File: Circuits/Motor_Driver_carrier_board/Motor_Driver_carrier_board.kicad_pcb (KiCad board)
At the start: 2 copper layers, 35 x 55.6 mm, 21 parts, among them P2 61301021021

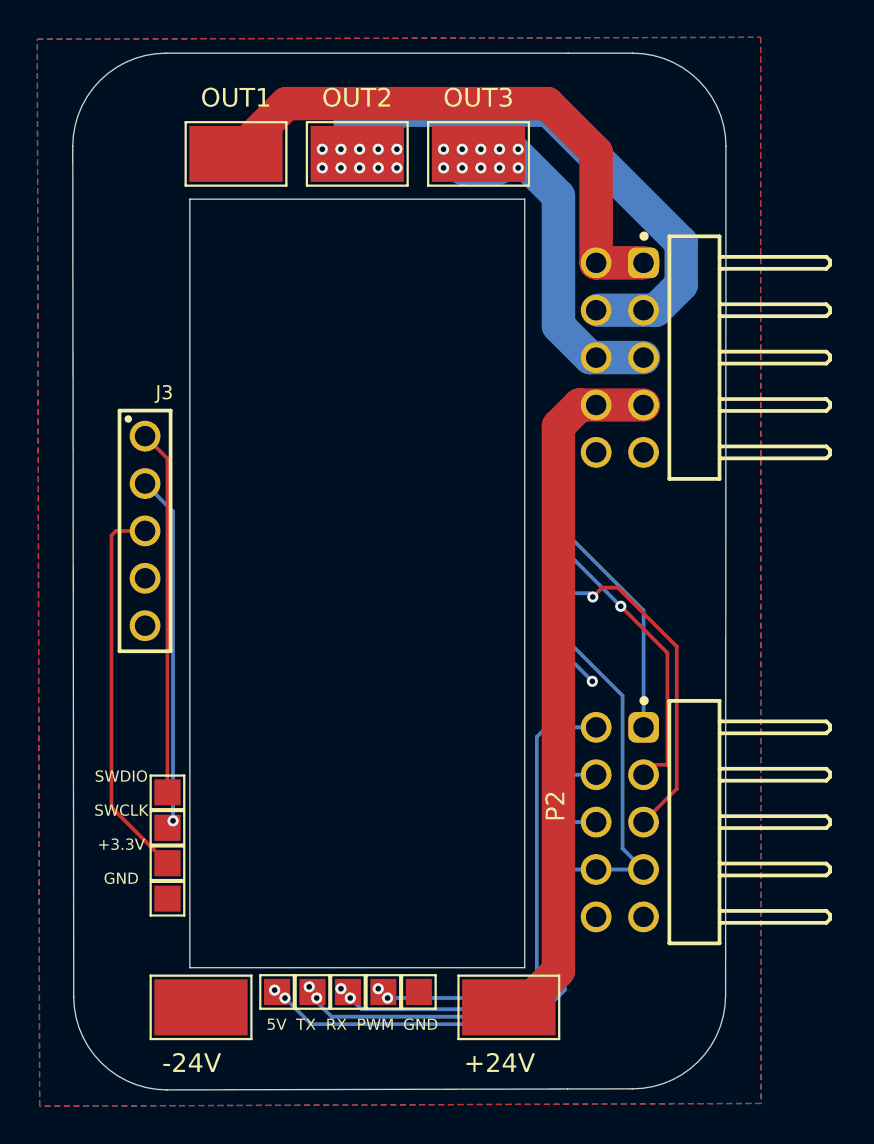
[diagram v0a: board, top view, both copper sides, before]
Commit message: Step file for mainboard pcb updated layout
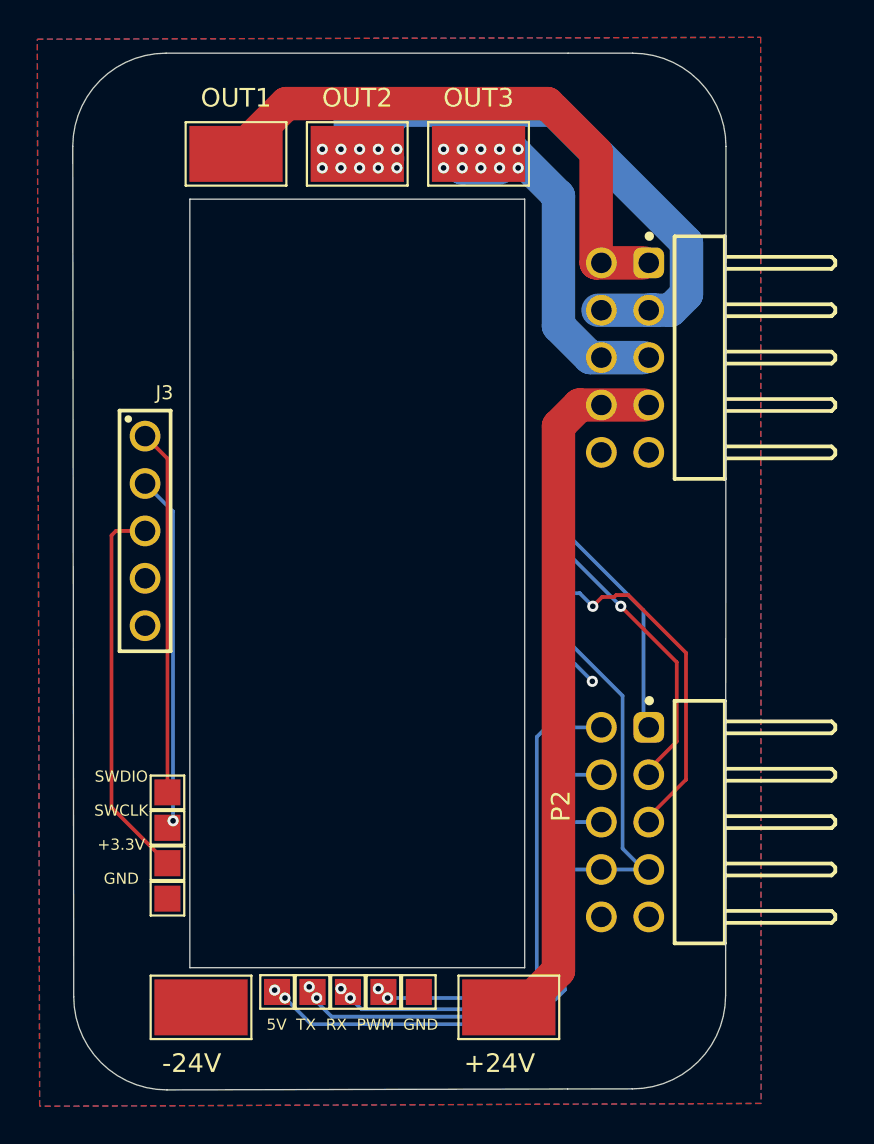
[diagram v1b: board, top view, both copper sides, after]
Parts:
- moved P2 0.28 mm to (151.2, 69.7)
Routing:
- net /OUT2: track 38.9 -> 40.2 mm
- net /H3: track 18.3 -> 18.8 mm
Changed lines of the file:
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@@
 	(footprint "61301021021:ESC_Adapter_pins_right_angle"
 		(layer "F.Cu")
-		(at 150.92 69.65 90)
+		(at 151.2 69.65 90)
 		(descr "Pin Header, pitch 2.54 mm, THT, Angled, dual row, 10p")
 		(property "Reference" "P2"
@@
 		)
 	)
-	(gr_rect
-		(start 118.85 41.34)
-		(end 153.89 97.2)
-		(stroke
-			(width 0.5)
-			(type default)
-		)
-		(fill none)
-		(layer "Eco1.User")
-	)
 	(gr_line
 		(start 148.92 97.07)
@@
 	)
 	(segment
-		(start 134.3 46.7)
-		(end 133.3 46.7)
+		(start 151.82083 54.475896)
+		(end 151.82083 51.711308)
+		(width 1.79166)
+		(layer "B.Cu")
+		(net 3)
+	)
+	(segment
+		(start 151.82083 51.711308)
+		(end 144.717862 44.60834)
 		(width 1.79166)
 		(layer "B.Cu")
@@
 	(segment
 		(start 134.3 46.7)
-		(end 136.39166 44.60834)
+		(end 133.3 46.7)
 		(width 1.79166)
 		(layer "B.Cu")
@@
 	)
 	(segment
-		(start 133.8 44.6)
-		(end 133.8 46.2)
+		(start 144.717862 44.60834)
+		(end 136.39166 44.60834)
 		(width 1.79166)
 		(layer "B.Cu")
@@
 	)
 	(segment
-		(start 151.54083 51.711308)
-		(end 151.54083 53.95917)
+		(start 134.3 46.7)
+		(end 136.39166 44.60834)
 		(width 1.79166)
 		(layer "B.Cu")
@@
 	)
 	(segment
-		(start 151.54083 53.95917)
-		(end 150.17 55.33)
+		(start 133.8 44.6)
+		(end 133.8 46.2)
 		(width 1.79166)
 		(layer "B.Cu")
@@
 	)
 	(segment
-		(start 144.437862 44.60834)
-		(end 151.54083 51.711308)
+		(start 150.966726 55.33)
+		(end 151.82083 54.475896)
 		(width 1.79166)
 		(layer "B.Cu")
@@
 	)
 	(segment
-		(start 136.39166 44.60834)
-		(end 144.437862 44.60834)
+		(start 149.8 55.33)
+		(end 150.966726 55.33)
 		(width 1.79166)
 		(layer "B.Cu")
@@
 	)
 	(segment
-		(start 150.8 79.7)
-		(end 150.05 79.7)
+		(start 151.3 74.2)
+		(end 151.3 78.45)
 		(width 0.2)
 		(layer "F.Cu")
@@
 	)
 	(segment
-		(start 148.3 71.2)
-		(end 150.8 73.7)
-		(width 0.2)
-		(layer "F.Cu")
-		(net 9)
-	)
-	(segment
-		(start 150.05 79.7)
+		(start 151.3 78.45)
 		(end 149.52 80.23)
 		(width 0.2)
@@
 	)
 	(segment
-		(start 150.8 73.7)
-		(end 150.8 79.7)
+		(start 148.3 71.2)
+		(end 151.3 74.2)
 		(width 0.2)
 		(layer "F.Cu")
@@
 	)
 	(segment
-		(start 146.8 70.7)
-		(end 147.3 70.2)
+		(start 148.7 70.6)
+		(end 151.8 73.7)
 		(width 0.2)
 		(layer "F.Cu")
@@
 	)
 	(segment
-		(start 148.148529 70.2)
-		(end 151.3 73.351471)
+		(start 148.051471 70.6)
+		(end 148.7 70.6)
 		(width 0.2)
 		(layer "F.Cu")
@@
 	)
 	(segment
-		(start 151.3 73.351471)
-		(end 151.3 80.99)
+		(start 151.8 73.7)
+		(end 151.8 80.49)
 		(width 0.2)
 		(layer "F.Cu")
@@
 	)
 	(segment
-		(start 147.3 70.2)
-		(end 148.148529 70.2)
+		(start 151.8 80.49)
+		(end 149.52 82.77)
 		(width 0.2)
 		(layer "F.Cu")
@@
 	)
 	(segment
-		(start 151.3 80.99)
-		(end 149.52 82.77)
+		(start 146.8 71.2)
+		(end 147.3 70.7)
+		(width 0.2)
+		(layer "F.Cu")
+		(net 12)
+	)
+	(segment
+		(start 147.951471 70.7)
+		(end 148.051471 70.6)
+		(width 0.2)
+		(layer "F.Cu")
+		(net 12)
+	)
+	(segment
+		(start 147.3 70.7)
+		(end 147.951471 70.7)
 		(width 0.2)
 		(layer "F.Cu")
@@
 	)
 	(via
-		(at 146.8 70.7)
+		(at 146.8 71.2)
 		(size 0.6)
 		(drill 0.3)
@@
 	)
 	(segment
-		(start 146.6 70.5)
-		(end 146.8 70.7)
+		(start 146.8 71.2)
+		(end 146.1 70.5)
 		(width 0.2)
 		(layer "B.Cu")
@@
 	)
 	(segment
-		(start 144.8 70.5)
-		(end 146.6 70.5)
+		(start 146.1 70.5)
+		(end 144.8 70.5)
 		(width 0.2)
 		(layer "B.Cu")
